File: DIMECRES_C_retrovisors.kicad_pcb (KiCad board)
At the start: 2 copper layers, 97.2 x 83.4 mm, 79 parts, among them J10 Vbat, J2 DE9_Pins, J3 Conn_01x05_Pin, J4 Motor3, J5 DE9_Pins, J6 Intermitente, J7 Calentador, J8 Motor2, J9 Motor1, Q1 DTC144E, Q2 DTC144E, Q3 DTC144E, SW1 SW_DPDT_G6S, SW10 SW_Push, SW2 SW_Push, SW3 SW_Push, SW4 SW_Push, SW5 SW_Push, SW6 SW_Push, SW7 SW_Push, SW8 FN01B, SW9 FN01B, U1 CH201, U10 LM1117DT-5.0, U2 ADM7160, U3 LM2596S-ADJ, U4 L298N, U5 TJA1042T, U6 ADA4511-2, U7 PIC18F4480-IP, Y1 Crystal

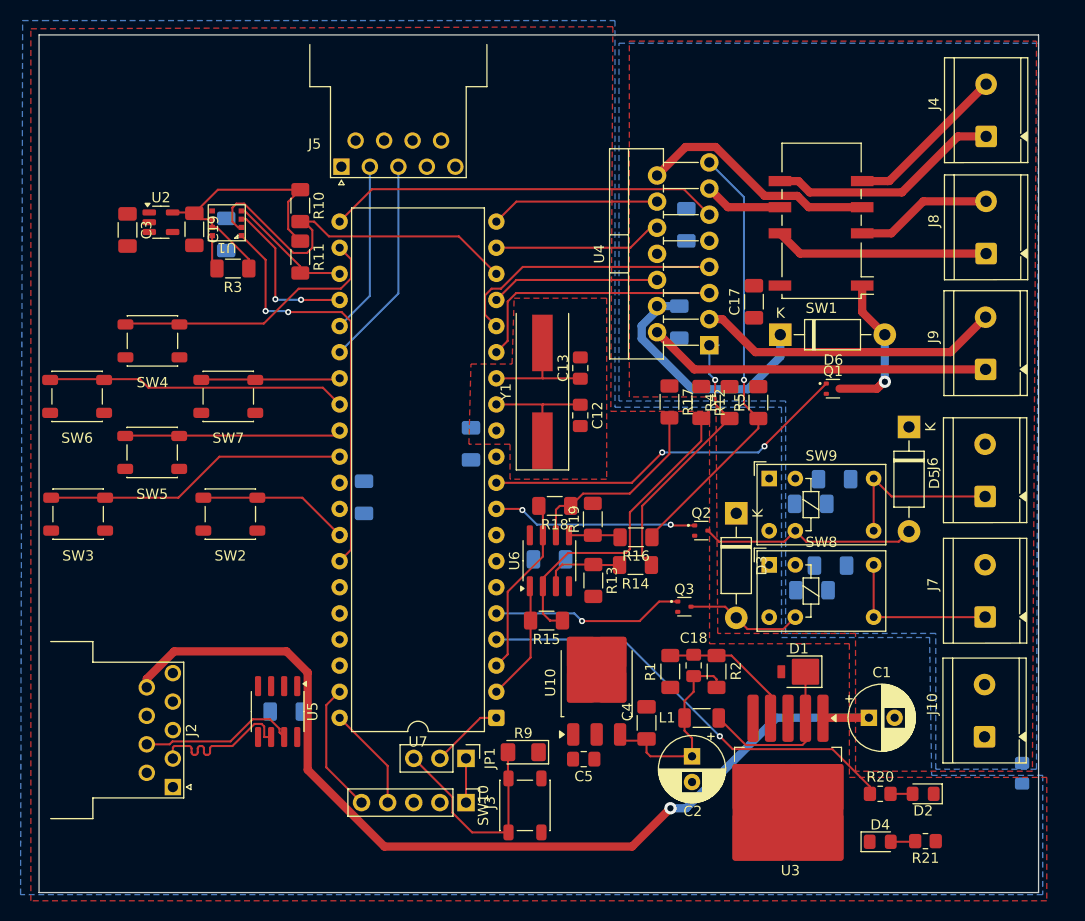
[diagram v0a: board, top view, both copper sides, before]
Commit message: Actu Layoutt
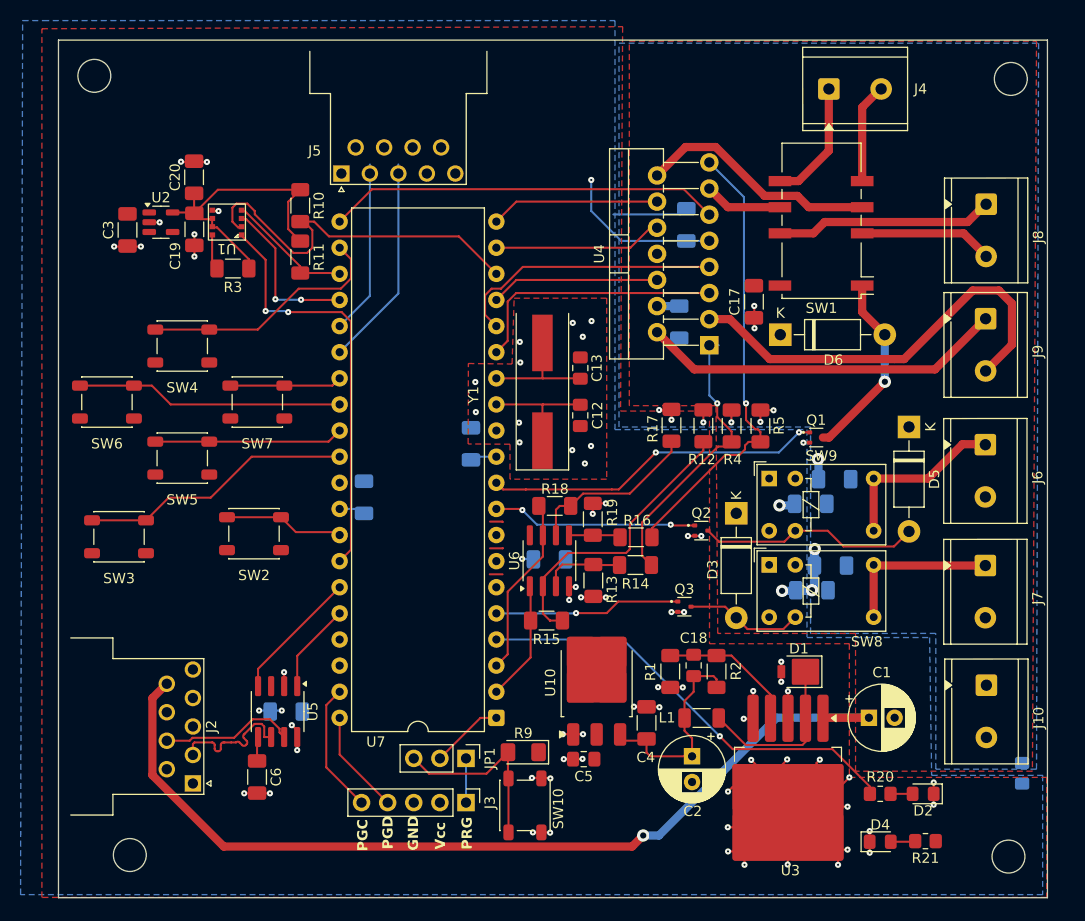
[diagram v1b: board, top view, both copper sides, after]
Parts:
- added C6: 47n, Capacitor_SMD:C_1206_3216Metric_Pad1.33x1.80mm_HandSolder, F.Cu at (108.2, 117.2)
- added REF**: MountingHole_3.2mm_M3, MountingHole:MountingHole_3.2mm_M3, F.Cu at (92.4, 49.0)
- added REF**: MountingHole_3.2mm_M3, MountingHole:MountingHole_3.2mm_M3, F.Cu at (95.8, 124.8)
- added REF**: MountingHole_3.2mm_M3, MountingHole:MountingHole_3.2mm_M3, F.Cu at (181.5, 49.3)
- added REF**: MountingHole_3.2mm_M3, MountingHole:MountingHole_3.2mm_M3, F.Cu at (181.3, 124.9)
- C20: moved to F.Cu
- moved J4 16.0 mm to (163.8, 50.2), turned to 0 degrees
- moved C20 6.38 mm to (102.1, 58.8), turned to 90 degrees
- moved J6 5.04 mm to (179.0, 84.8), turned to -90 degrees
- moved Q1 5.02 mm to (162.6, 84.2)
- moved J10 5.02 mm to (179.1, 108.2), turned to -90 degrees
- moved J7 5.01 mm to (179.0, 96.6), turned to -90 degrees
- moved J9 4.93 mm to (179.1, 72.6), turned to -90 degrees
- moved J8 4.80 mm to (179.1, 61.5), turned to -90 degrees
- moved SW3 4.54 mm to (94.8, 93.8)
- moved SW2 2.98 mm to (107.9, 93.5)
- moved SW5 2.98 mm to (100.9, 86.2)
- moved SW6 2.95 mm to (93.6, 80.7)
- moved SW4 2.94 mm to (100.9, 75.2)
- moved SW7 2.88 mm to (108.2, 80.7)
- moved R5 2.28 mm to (157.2, 83.0)
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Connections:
- net Net-(J6-Pin_1) renamed /M_Inter
- net Net-(J7-Pin_1) renamed /M_calen
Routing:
- net GND: track 0.00 -> 102.3 mm, vias 0 -> 69
- net Vcc: track 0.00 -> 28.6 mm, vias 0 -> 4
- net Vbat: track 120.0 -> 103.9 mm, vias 1 -> 6
- net CANTX: track 0.00 -> 12.9 mm
- net /Motor1B: track 29.6 -> 42.2 mm
- net /Motor3A: track 22.8 -> 12.0 mm
- net GNDPWR: track 0.00 -> 9.38 mm, vias 0 -> 8
- net CANRX: track 0.00 -> 8.78 mm
- net /Motor3B: track 16.0 -> 9.77 mm
- net B_Left: track 29.2 -> 26.0 mm
- net Act_Rele_M2/M3: track 36.1 -> 33.0 mm
- net B_Un/Fold: track 14.8 -> 11.7 mm
- net B_Heat: track 29.7 -> 26.6 mm
- net /M_D: track 15.7 -> 18.6 mm
- net B_Down: track 21.0 -> 18.4 mm
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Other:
- board size 97.2 x 83.4 mm -> 96.2 x 83.4 mm
- board text added: "GND"
- board text added: "PGC"
- board text added: "PGD"
- board text added: "PRG"
- board text added: "Vcc"

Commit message: .,.,-
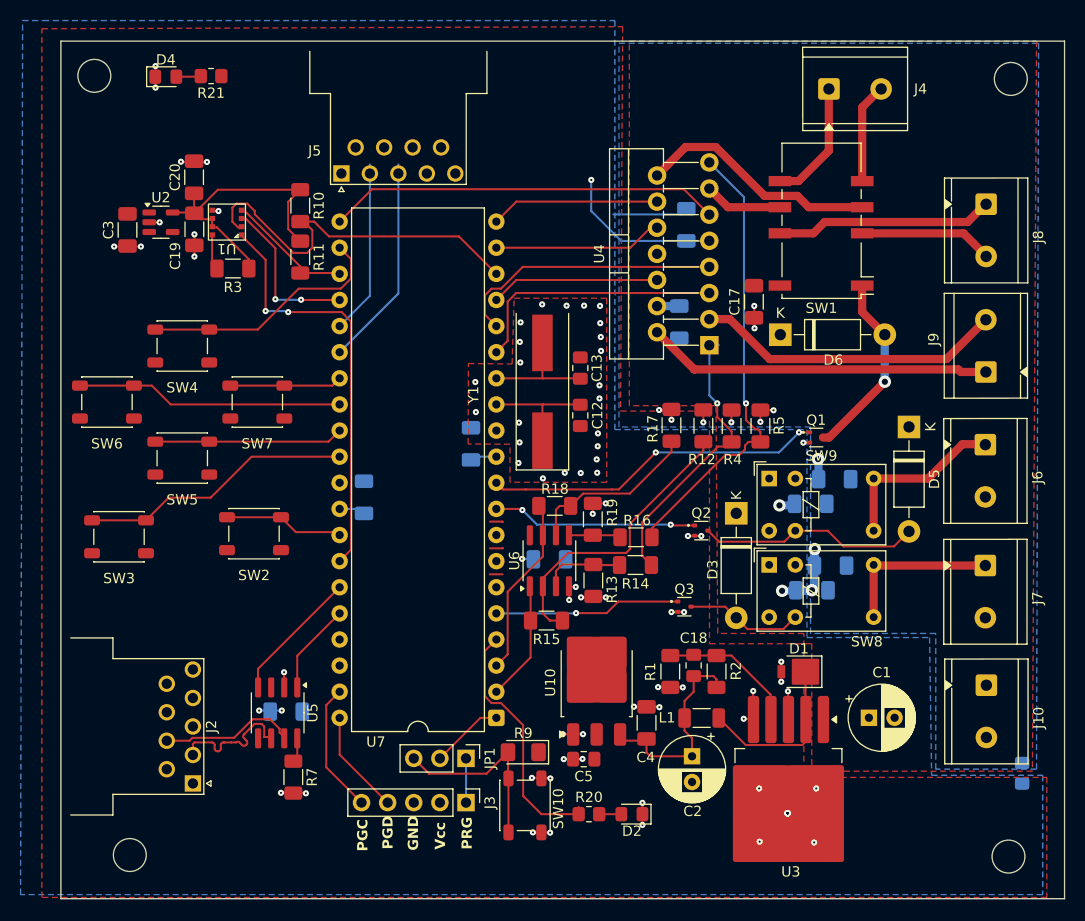
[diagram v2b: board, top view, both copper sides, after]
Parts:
- removed C6: 47n, Capacitor_SMD:C_1206_3216Metric_Pad1.33x1.80mm_HandSolder
- added R7: 15k, Resistor_SMD:R_1206_3216Metric_Pad1.30x1.75mm_HandSolder, F.Cu at (111.7, 117.2)
- U5: value TJA1042T -> MCP2551-I-SN
- moved D4 101.8 mm to (99.3, 49.1)
- moved R21 101.8 mm to (103.7, 49.0)
- moved R20 28.4 mm to (140.5, 120.8)
- moved D2 28.4 mm to (144.7, 120.8)
- moved J9 5.18 mm to (179.1, 77.8), turned to 90 degrees
- moved U3 0.13 mm to (159.9, 119.2)
- moved U5 0.13 mm to (110.2, 110.9)
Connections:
- C22 pad 1: Vbat -> Vcc
- C22 pad 2: GNDPWR -> GND
- D3 pad 1: Vbat -> Vcc
- SW8 pad 3: Vbat -> Vcc
- U5 pad 5: Net-(U5-SPLIT) -> unconnected-(U5-Vref-Pad5)
- U5 pad 8: GND -> Net-(U5-Rs)
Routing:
- net Vbat: track 103.9 -> 12.3 mm, vias 6 -> 5
- net GND: track 102.3 -> 55.3 mm, vias 69 -> 76
- net AngleMort: track 43.0 -> 24.6 mm, vias 1 -> 0
- net /Motor1B: track 42.2 -> 30.1 mm
- net Net-(U5-Rs): track 0.00 -> 3.01 mm
- net Net-(U5-SPLIT): track 2.36 -> 0.00 mm
- net /Motor1A: track 35.5 -> 33.6 mm
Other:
- board size 96.2 x 83.4 mm -> 97.6 x 83.4 mm
